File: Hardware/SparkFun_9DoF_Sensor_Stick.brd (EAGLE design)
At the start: 34.3 x 10.2 mm, 27 parts, among them U1 ITG-32001:1, U2 ADXL345, U4 3.3V

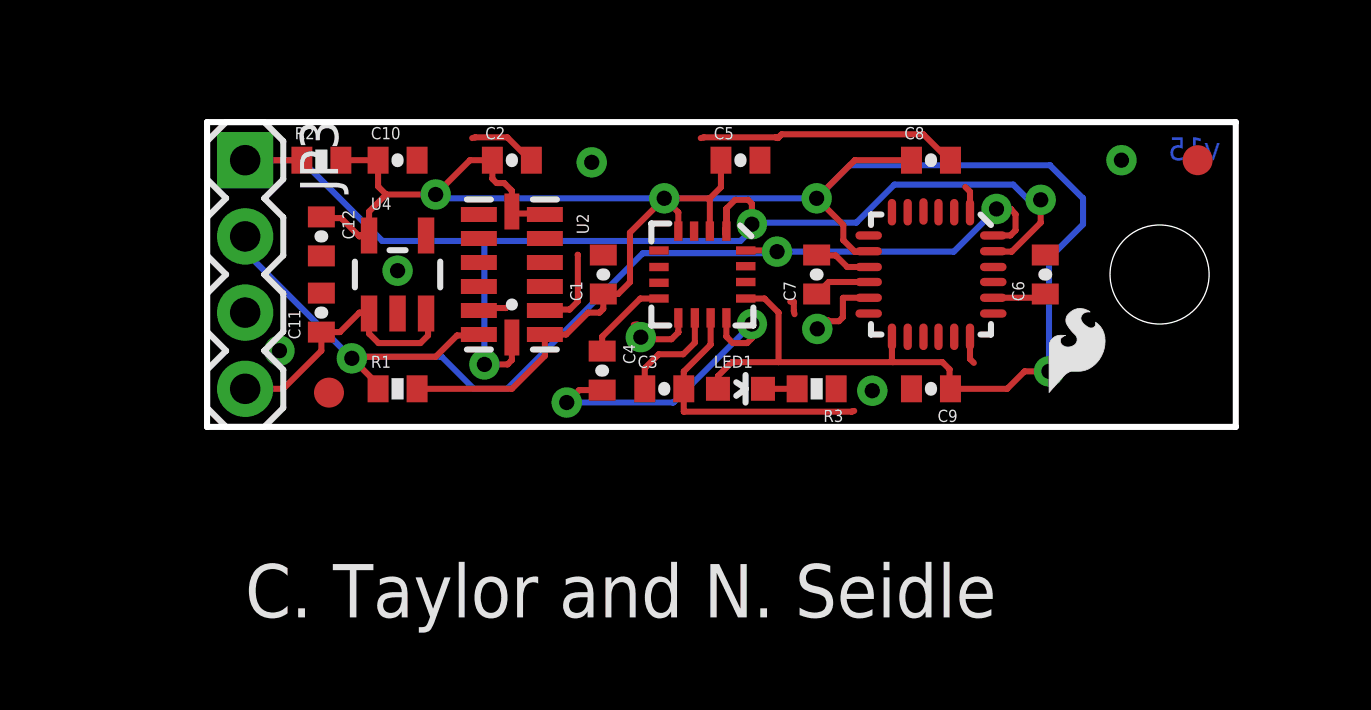
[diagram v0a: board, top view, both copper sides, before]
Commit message: Mid revision work - NOT FUNCTIONAL
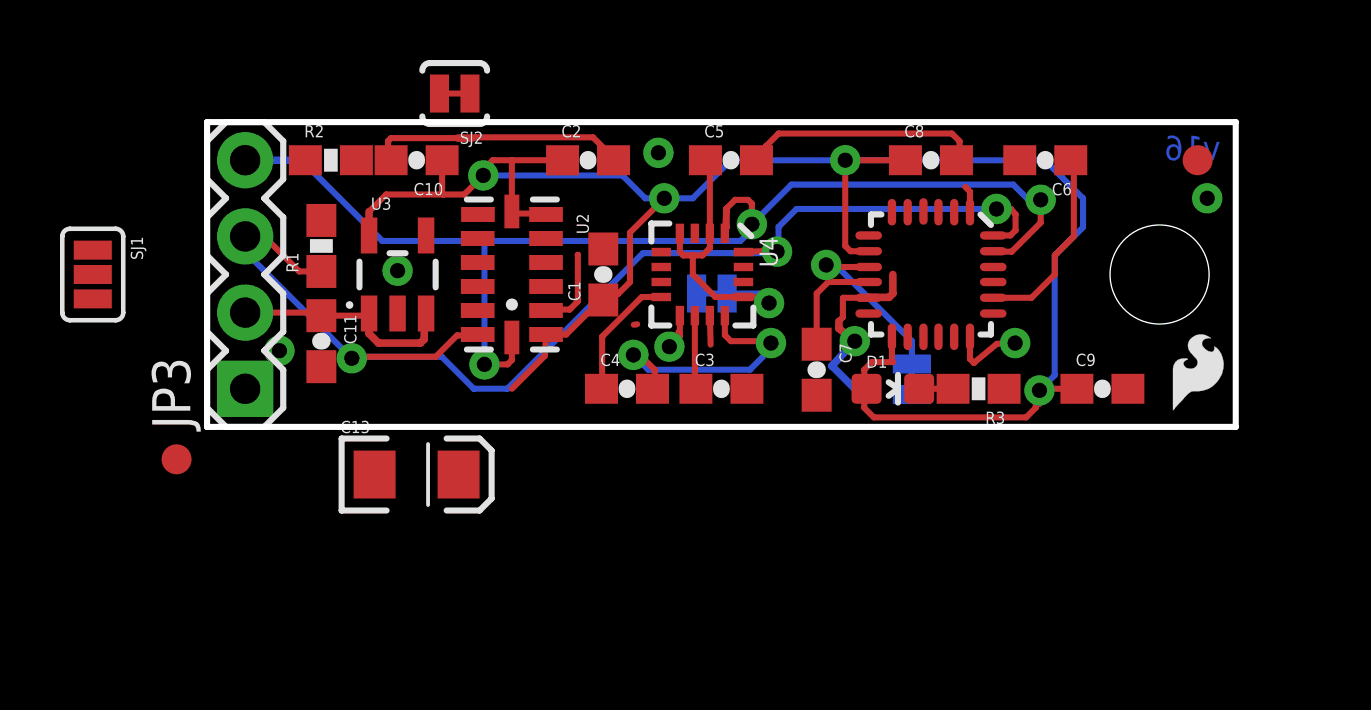
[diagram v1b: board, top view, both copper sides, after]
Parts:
- removed C12: 4.7uF, SparkFun:0402-CAP
- removed LED1: Blue, SparkFun:LED-0603
- removed U$1: CREATIVE_COMMONS, SparkFun:CREATIVE_COMMONS
- removed U$2: HMC5883L1:1, Testing:16LPCC_1:1
- added C13: 10uF, SparkFun-Capacitors:EIA3216
- added D1: RED, SparkFun-LED:LED-0603
- added FRAME1: (no value), SparkFun-Aesthetics:CREATIVE_COMMONS
- added SJ1: JUMPER-PAD-3-NC_BY_PASTE, SparkFun-Passives:PAD-JUMPER-3-NC_BY_PASTE_YES_SILK_FULL_BOX
- added SJ2, SJ3, SJ4: JUMPER-PAD-2-NC_BY_TRACE, SparkFun-Passives:PAD-JUMPER-2-NC_BY_TRACE_YES_SILK
- added U$4: REVISION, SparkFun-Aesthetics:REVISION
- added U3: 3.3V/150mA, SparkFun-PowerIC:SOT23-5
- C1, C10, C11, C2, C3, C4, C5, C6, C7, C8, C9: device SparkFun:0402-CAP -> SparkFun-Capacitors:0603-CAP
- JP1, JP2: device SparkFun:FIDUCIAL-1X2 -> SparkFun-Aesthetics:FIDUCIAL-1X2
- JP3: device SparkFun:1X04 -> SparkFun-Connectors:1X04
- JP4: value LOGO-SFESK -> SFE_LOGO_FLAME.1_INCH; device SparkFun:SFE-LOGO-FLAME -> SparkFun-Aesthetics:SFE_LOGO_FLAME_.1
- JP5: device SparkFun:STAND-OFF -> SparkFun-Electromechanical:STAND-OFF
- R1, R2, R3: device SparkFun:0402-RES -> SparkFun-Resistors:0603-RES
- U$3: device SparkFun:OSHW-LOGO-S -> SparkFun-Aesthetics:OSHW-LOGO-S
- U1: device Testing:QFN-24_1:1 -> SparkFun-Sensors:QFN-24_ITG3200_1:1
- U2: value ADXL345 -> ADXL345"; device SparkFun:LGA14 -> SparkFun-Sensors:ADXL3451:1
- U4: value 3.3V -> HMC5883LSMD; device SparkFun:SOT23-5 -> SparkFun-Sensors:16LPCC
- moved U4 10.2 mm to (16.5, 5.08), turned to 270 degrees
- moved JP3 7.62 mm to (1.27, 1.27), turned to 90 degrees
- moved C9 5.71 mm to (29.8, 1.27), turned to 0 degrees
- moved JP2 5.54 mm to (-1.02, -1.08)
- moved R3 5.40 mm to (25.7, 1.27)
- moved R1 5.40 mm to (3.81, 6.03), turned to 90 degrees
- moved U$3 4.02 mm to (31.1, 12.1)
- moved JP4 3.93 mm to (31.9, 0.19)
- moved C6 3.81 mm to (27.9, 8.89), turned to 180 degrees
- moved C7 3.17 mm to (20.3, 1.91), turned to 270 degrees
- moved C2 2.54 mm to (12.7, 8.89)
- moved C3 1.90 mm to (17.1, 1.27)
- moved C4 1.03 mm to (14.0, 1.27), turned to 0 degrees
- moved C11 0.95 mm to (3.81, 2.86), turned to 270 degrees
- moved C10 0.64 mm to (6.99, 8.89), turned to 180 degrees
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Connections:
- new net N$10: SJ2.2, U2.12
- new net N$12: C5.1, SJ4.2, U4.13, U4.2, U4.4
- new net N$6: R1.2, SJ1.3
- new net N$8: R2.2, SJ1.1
- new net N$9: SJ3.2, U1.9
- net 3.3V: now also C13.A, D1.A, SJ1.2, SJ4.1, U3.5; no longer C12.1, C5.1, LED1.A, R1.2, R2.2, U$2.13, U$2.2, U$2.4, U4.5
- net GND: now also C13.C, JP3.1, SJ2.1, SJ3.1, U3.2, U4.11, U4.9; no longer C12.2, JP3.3, U$2.11, U$2.9, U1.9, U2.12, U4.2
- net N$1: now also U4.10; no longer U$2.10
- net N$2: now also U4.8; no longer U$2.8
- net N$3: now also U4.12; no longer U$2.12
- net N$4: now also D1.C; no longer LED1.C
- net SCL: now also JP3.4, U4.1; no longer JP3.1, U$2.1
- net SDA: now also JP3.3, U4.16; no longer JP3.2, U$2.16
- net VCC: now also JP3.2, U3.1, U3.3; no longer JP3.4, U4.1, U4.3
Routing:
- net 3.3V: track 82.9 -> 67.0 mm
- net N$12: track 0.00 -> 9.86 mm, vias 0 -> 1
- net N$9: track 0.00 -> 6.12 mm, vias 0 -> 1
- net N$5: track 1.93 -> 6.49 mm
- net SDA: track 39.1 -> 41.2 mm
- net SCL: track 42.7 -> 40.9 mm
- net N$7: track 1.90 -> 3.58 mm
- net N$3: track 10.7 -> 9.15 mm
- net VCC: track 9.19 -> 7.78 mm
- net N$2: track 2.90 -> 4.27 mm
- net N$1: track 3.53 -> 2.45 mm
- net GND: track 32.5 -> 31.8 mm
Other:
- board text added: "Toni Klopfenstein"
- board text added: "v16"
- board text removed: "v15"
